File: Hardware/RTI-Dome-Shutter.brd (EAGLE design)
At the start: 80 x 71.1 mm, 42 parts, among them IC1 24AA128ST, IC5 74LVC245, IC6 74ABT245, J1 POWERPOLE_POWER45A

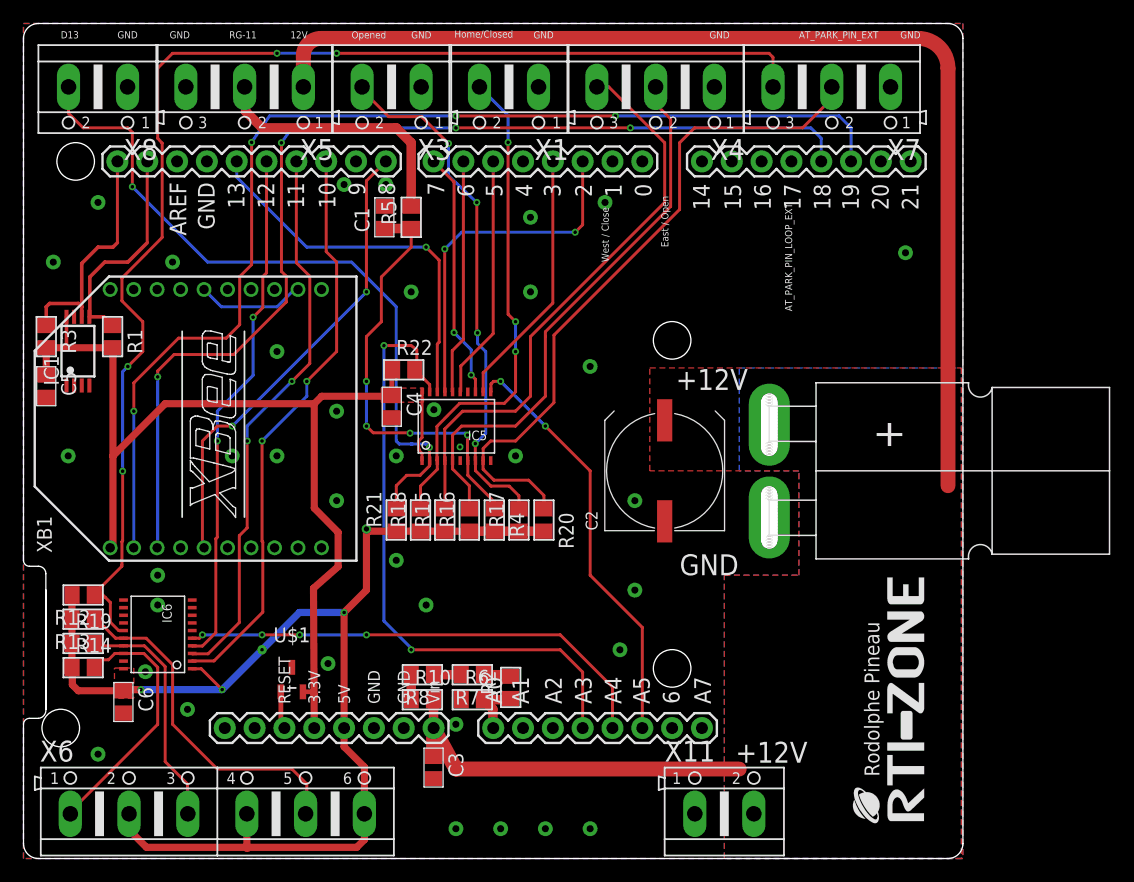
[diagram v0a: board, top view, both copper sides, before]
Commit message: Fix some componenent manufacturer reference
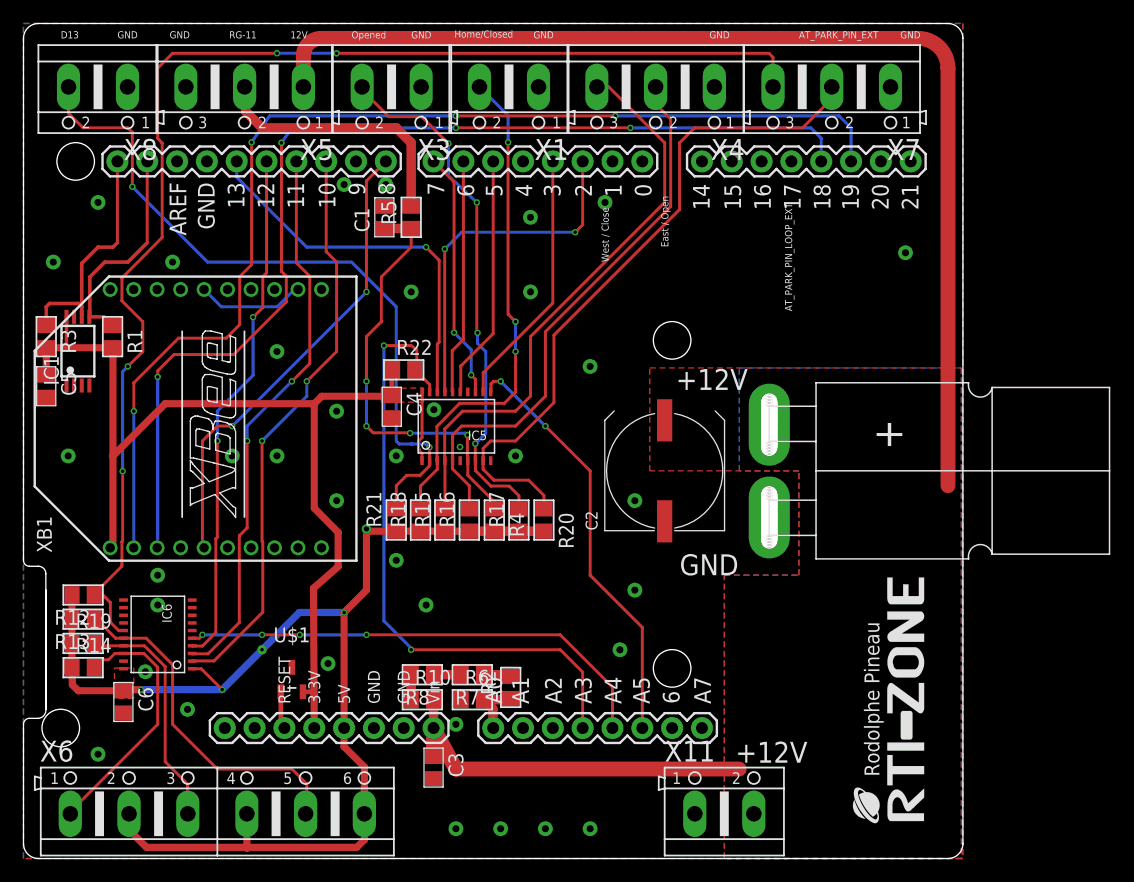
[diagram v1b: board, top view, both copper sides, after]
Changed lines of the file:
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@@
 </class>
 </classes>
-<designrules name="Fusion">
-<description language="de">&lt;b&gt;EAGLE Design Rules&lt;/b&gt;
+<designrules name="jlcpcb2layer">
+<description language="en">&lt;b&gt;JLCPCB Design Rules by Jaap de Dood&lt;/b&gt;
 &lt;p&gt;
-Die Standard-Design-Rules sind so gewÃÂÃÂ¤hlt, dass sie fÃÂÃÂ¼r
-die meisten Anwendungen passen. Sollte ihre Platine
-besondere Anforderungen haben, treffen Sie die erforderlichen
-Einstellungen hier und speichern die Design Rules unter
-einem neuen Namen ab.</description>
-<description language="en">&lt;b&gt;EAGLE Design Rules&lt;/b&gt;
-&lt;p&gt;
-The default Design Rules have been set to cover
-a wide range of applications. Your particular design
-may have different requirements, so please make the
-necessary adjustments and save your customized
-design rules under a new name.</description>
+Please make sure your boards conform to these design rules.
+&lt;/p&gt;</description>
 <param name="layerSetup" value="(1*16)"/>
-<param name="mtCopper" value="0.07mm 0.035mm 0.035mm 0.035mm 0.035mm 0.035mm 0.035mm 0.035mm 0.035mm 0.035mm 0.035mm 0.035mm 0.035mm 0.035mm 0.035mm 0.07mm"/>
-<param name="mtIsolate" value="1.6mm 0.5mm 0.25mm 0.15mm 0.2mm 0.15mm 0.2mm 0.15mm 0.2mm 0.15mm 0.2mm 0.15mm 0.2mm 0.25mm 0.5mm"/>
-<param name="mdWireWire" value="8mil"/>
-<param name="mdWirePad" value="8mil"/>
-<param name="mdWireVia" value="8mil"/>
-<param name="mdPadPad" value="8mil"/>
-<param name="mdPadVia" value="8mil"/>
-<param name="mdViaVia" value="8mil"/>
-<param name="mdSmdPad" value="6mil"/>
-<param name="mdSmdVia" value="6mil"/>
-<param name="mdSmdSmd" value="6mil"/>
+<param name="mtCopper" value="0.035mm 0.035mm 0.035mm 0.035mm 0.035mm 0.035mm 0.035mm 0.035mm 0.035mm 0.035mm 0.035mm 0.035mm 0.035mm 0.035mm 0.035mm 0.035mm"/>
+<param name="mtIsolate" value="1.6mm 0.15mm 0.2mm 0.15mm 0.2mm 0.15mm 0.2mm 0.15mm 0.2mm 0.15mm 0.2mm 0.15mm 0.2mm 0.15mm 0.2mm"/>
+<param name="mdWireWire" value="5mil"/>
+<param name="mdWirePad" value="5mil"/>
+<param name="mdWireVia" value="5mil"/>
+<param name="mdPadPad" value="5mil"/>
+<param name="mdPadVia" value="5mil"/>
+<param name="mdViaVia" value="5mil"/>
+<param name="mdSmdPad" value="5mil"/>
+<param name="mdSmdVia" value="5mil"/>
+<param name="mdSmdSmd" value="5mil"/>
 <param name="mdViaViaSameLayer" value="8mil"/>
 <param name="mnLayersViaInSmd" value="2"/>
-<param name="mdCopperDimension" value="13mil"/>
-<param name="mdDrill" value="6mil"/>
+<param name="mdCopperDimension" value="8mil"/>
+<param name="mdDrill" value="0.5mm"/>
 <param name="mdSmdStop" value="0mil"/>
-<param name="msWidth" value="8mil"/>
-<param name="msDrill" value="0.3mm"/>
-<param name="msMicroVia" value="8mil"/>
+<param name="msWidth" value="5mil"/>
+<param name="msDrill" value="0.2mm"/>
+<param name="msMicroVia" value="0.2mm"/>
 <param name="msBlindViaRatio" value="0.5"/>
 <param name="rvPadTop" value="0.25"/>
@@
 <param name="rvMicroViaOuter" value="0.25"/>
 <param name="rvMicroViaInner" value="0.25"/>
-<param name="rlMinPadTop" value="6mil"/>
+<param name="rlMinPadTop" value="0.13mm"/>
 <param name="rlMaxPadTop" value="20mil"/>
-<param name="rlMinPadInner" value="6mil"/>
+<param name="rlMinPadInner" value="0.13mm"/>
 <param name="rlMaxPadInner" value="20mil"/>
-<param name="rlMinPadBottom" value="6mil"/>
+<param name="rlMinPadBottom" value="0.13mm"/>
 <param name="rlMaxPadBottom" value="20mil"/>
-<param name="rlMinViaOuter" value="6mil"/>
+<param name="rlMinViaOuter" value="0.13mm"/>
 <param name="rlMaxViaOuter" value="20mil"/>
-<param name="rlMinViaInner" value="6mil"/>
+<param name="rlMinViaInner" value="0.13mm"/>
 <param name="rlMaxViaInner" value="20mil"/>
-<param name="rlMinMicroViaOuter" value="6mil"/>
+<param name="rlMinMicroViaOuter" value="0.13mm"/>
 <param name="rlMaxMicroViaOuter" value="20mil"/>
-<param name="rlMinMicroViaInner" value="6mil"/>
+<param name="rlMinMicroViaInner" value="0.13mm"/>
 <param name="rlMaxMicroViaInner" value="20mil"/>
 <param name="psTop" value="-1"/>
@@
 <param name="mvStopFrame" value="1"/>
 <param name="mvCreamFrame" value="0"/>
-<param name="mlMinStopFrame" value="3mil"/>
-<param name="mlMaxStopFrame" value="3mil"/>
-<param name="mlMinCreamFrame" value="0mil"/>
+<param name="mlMinStopFrame" value="0.05mm"/>
+<param name="mlMaxStopFrame" value="2.5mil"/>
+<param name="mlMinCreamFrame" value="0.05mm"/>
 <param name="mlMaxCreamFrame" value="0mil"/>
-<param name="mlViaStopLimit" value="130mil"/>
+<param name="mlViaStopLimit" value="40mil"/>
 <param name="srRoundness" value="0"/>
 <param name="srMinRoundness" value="0mil"/>
 <param name="srMaxRoundness" value="0mil"/>
-<param name="slThermalIsolate" value="8mil"/>
+<param name="slThermalIsolate" value="10mil"/>
 <param name="slThermalsForVias" value="0"/>
 <param name="dpMaxLengthDifference" value="10mm"/>
@@
 <param name="checkFont" value="1"/>
 <param name="checkRestrict" value="1"/>
-<param name="useDiameter" value="31"/>
+<param name="useDiameter" value="13"/>
 <param name="maxErrors" value="50"/>
 </designrules>
